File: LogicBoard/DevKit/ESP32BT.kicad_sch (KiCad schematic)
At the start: 20 parts, among them J13 USBC Socket, J15 ESPUartConn, J17 MicroSD, U10 ESP32-C3-WROOM-02-N4, U8 USBLC6-2SC6

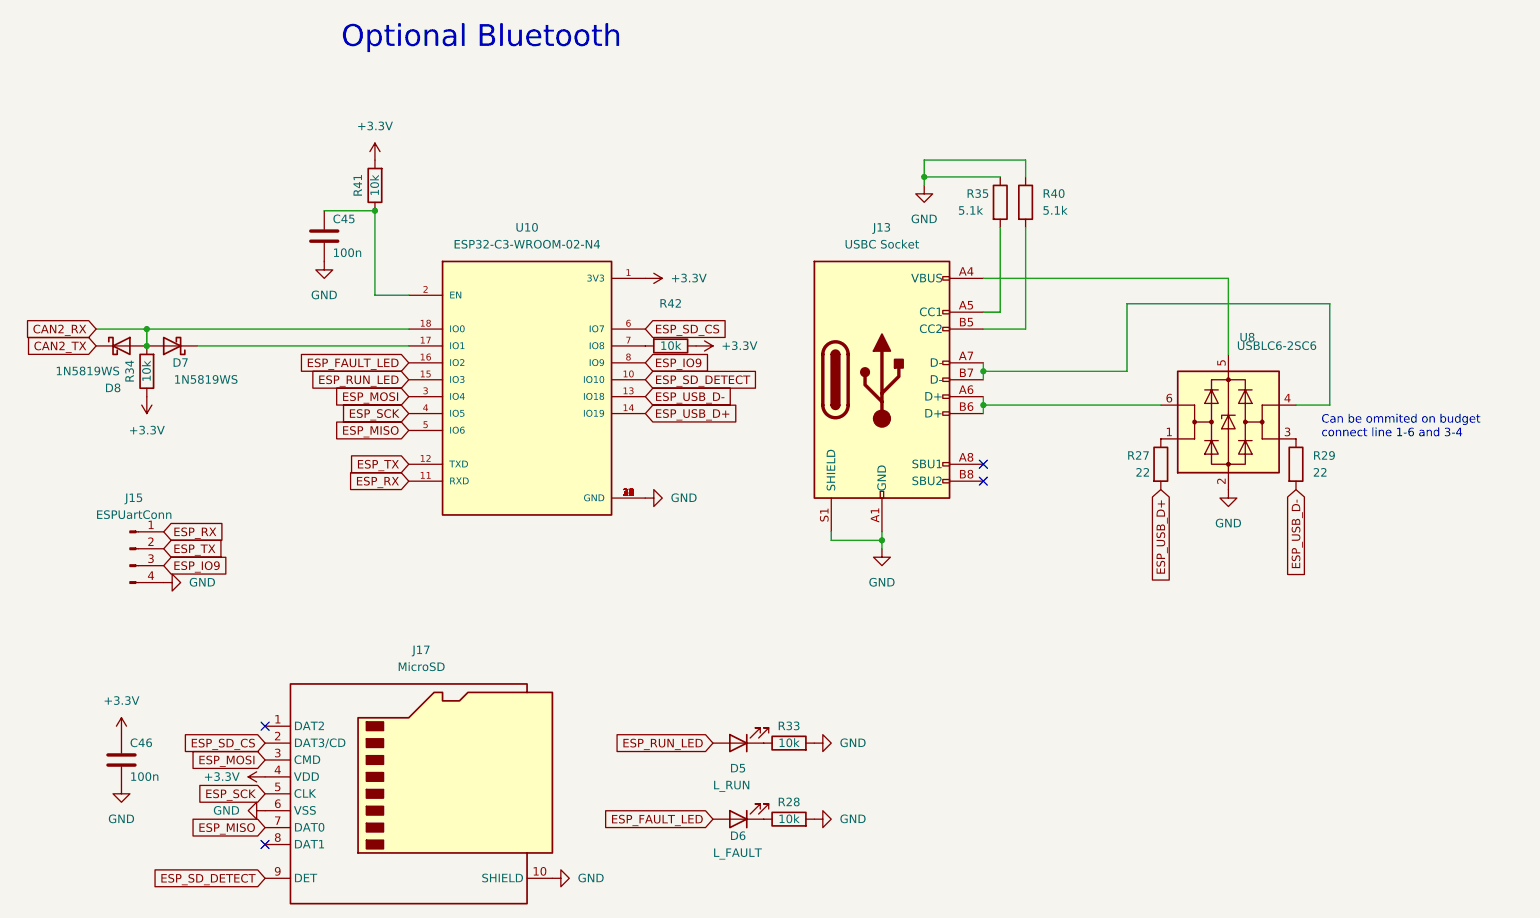
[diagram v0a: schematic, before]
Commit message: v3.2.2 - TL494V2
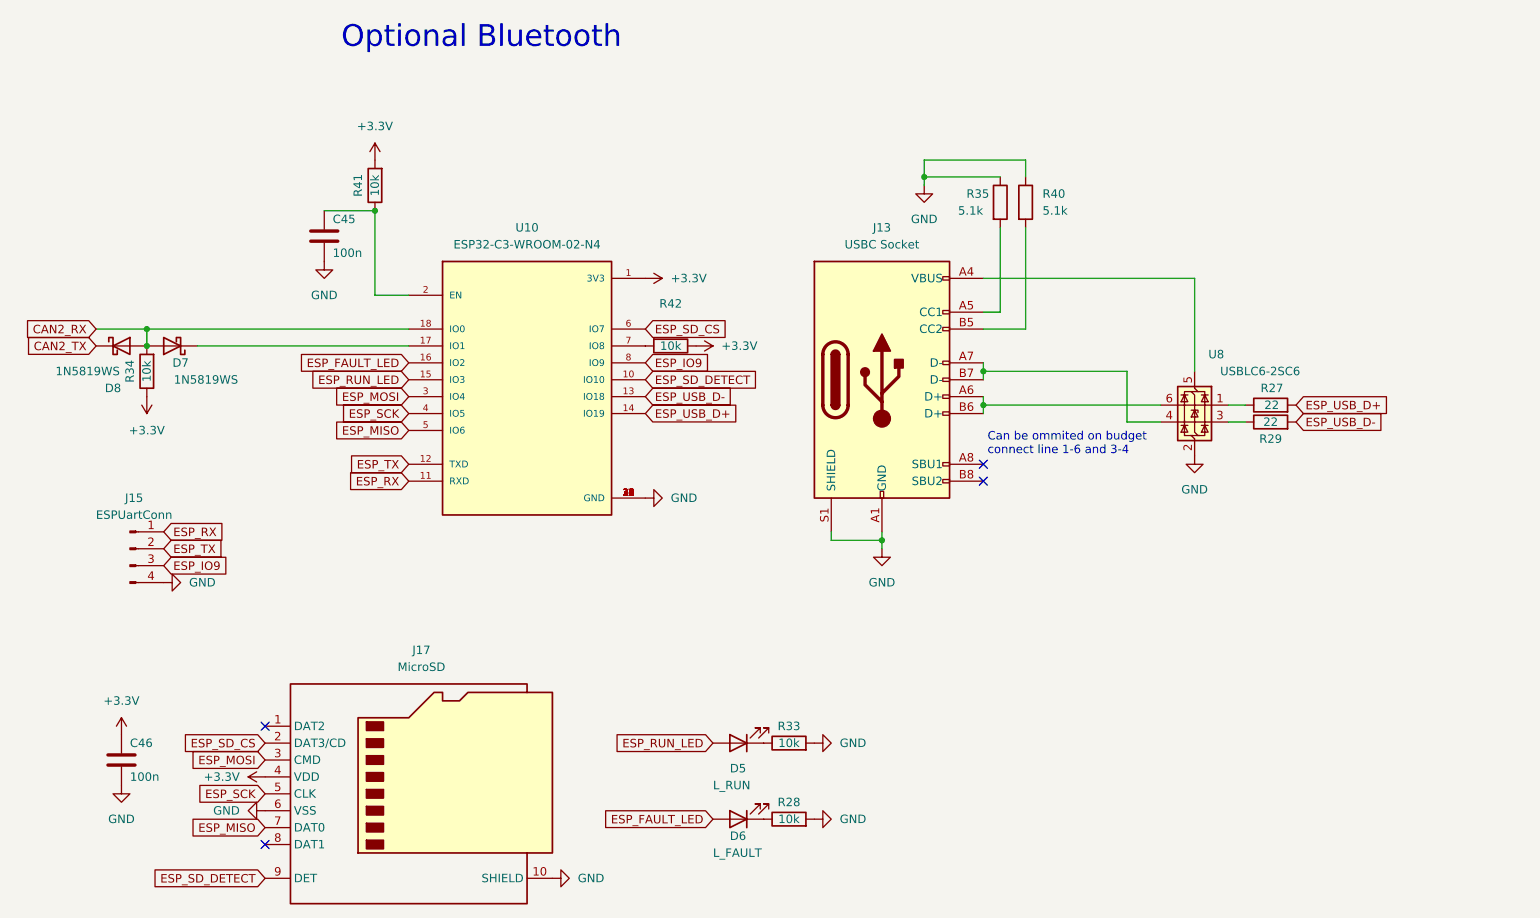
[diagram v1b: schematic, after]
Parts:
- removed J13: USBC Socket, Connector_USB:USB_C_Receptacle_GCT_USB4105-xx-A_16P_TopMnt_Horizontal, symbol Connector:USB_C_Receptacle_USB2.0
- removed U8: USBLC6-2SC6, Package_TO_SOT_SMD:SOT-23-6, symbol Power_Protection:USBLC6-2P6
- added J13: USBC Socket, Connector_USB:USB_C_Receptacle_GCT_USB4105-xx-A_16P_TopMnt_Horizontal, symbol Connector:USB_C_Receptacle_USB2.0_16P
- added U8: USBLC6-2SC6, Package_TO_SOT_SMD:SOT-23-6, symbol Power_Protection:USBLC6-2SC6
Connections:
- net GND: now also J13.A1 (GND), J13.A12 (GND), J13.B1 (GND), J13.B12 (GND), J13.S1 (SHIELD), U8.2 (GND)
- net at R40.2: now also J13.B5 (CC2)
- net at R35.2: now also J13.A5 (CC1)
- net at R27.1: now also U8.1 (I/O1)
- net at R29.1: now also U8.3 (I/O2)
- new net: J13.A7 (D-), J13.B7 (D-), U8.4 (I/O2)
- new net: J13.A4 (VBUS), J13.A9 (VBUS), J13.B4 (VBUS), J13.B9 (VBUS), U8.5 (VBUS)
- new net: J13.A6 (D+), J13.B6 (D+), U8.6 (I/O1)
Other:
- moved on the sheet: R27, R29
